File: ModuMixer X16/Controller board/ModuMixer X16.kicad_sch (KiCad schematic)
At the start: 0 parts

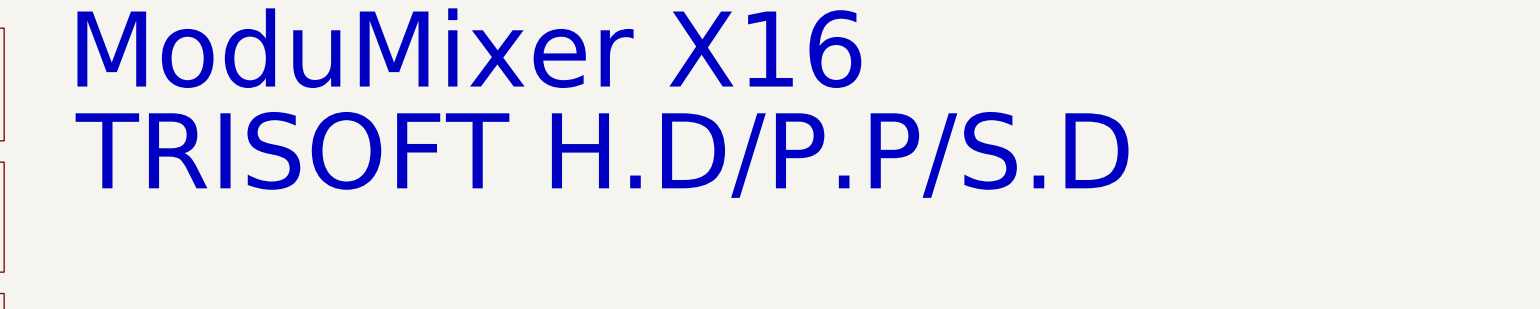
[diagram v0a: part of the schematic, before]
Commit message: idk testing github desktop
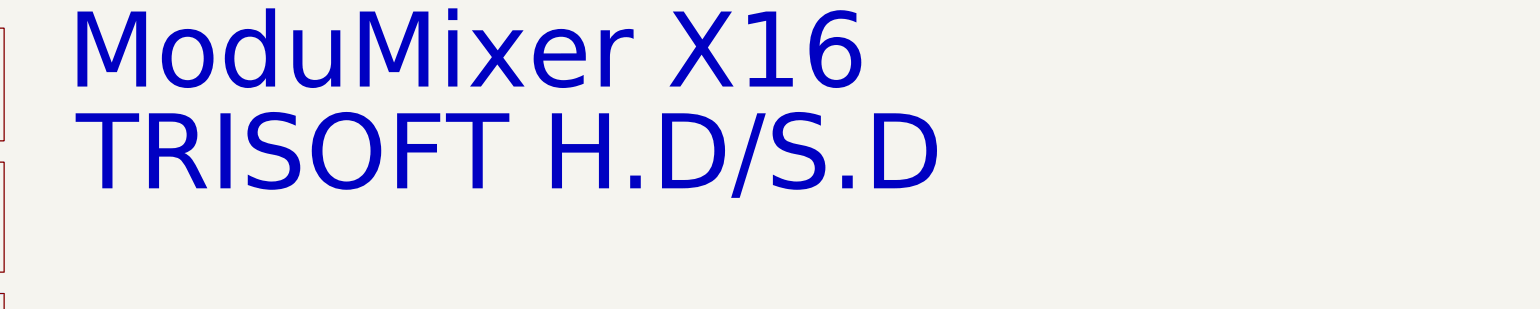
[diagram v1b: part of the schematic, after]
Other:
- note added: "TRISOFT H.D/S.D CONFIDENTIAL DO NOT SHARE"
- note removed: "TRISOFT H.D/P.P/S.D CONFIDENTIAL DO NOT SHARE"
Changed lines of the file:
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@@
 		)
 	)
-	(text "TRISOFT H.D/P.P/S.D\n\nCONFIDENTIAL\nDO NOT SHARE"
+	(text "TRISOFT H.D/S.D\n\nCONFIDENTIAL\nDO NOT SHARE"
 		(exclude_from_sim no)
 		(at 11.938 90.678 0)
